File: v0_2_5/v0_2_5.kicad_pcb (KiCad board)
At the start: 2 copper layers, 91.4 x 50.8 mm, 58 parts, among them IC1 RASPBERRY_PI_PICO_W, IC2 BH1750FVI-TR, IC3 AP2138N-3.3TRG1, J1 S2B-PH-SM4-TB_LF__SN_, J2 HYCW110-TF10-180B, J4 SM04B-SRSS-TB, J5 Screw_Terminal_01x03, J6 Conn_01x02_Pin, Q1 DMG2301L-7, Q2 DMG2301L-7, Q3 DMG2301L-7, Q5 DMN3731U-7, U1 AHT20, U2 PCF85063ATL, Y1 Q13FC1350000200

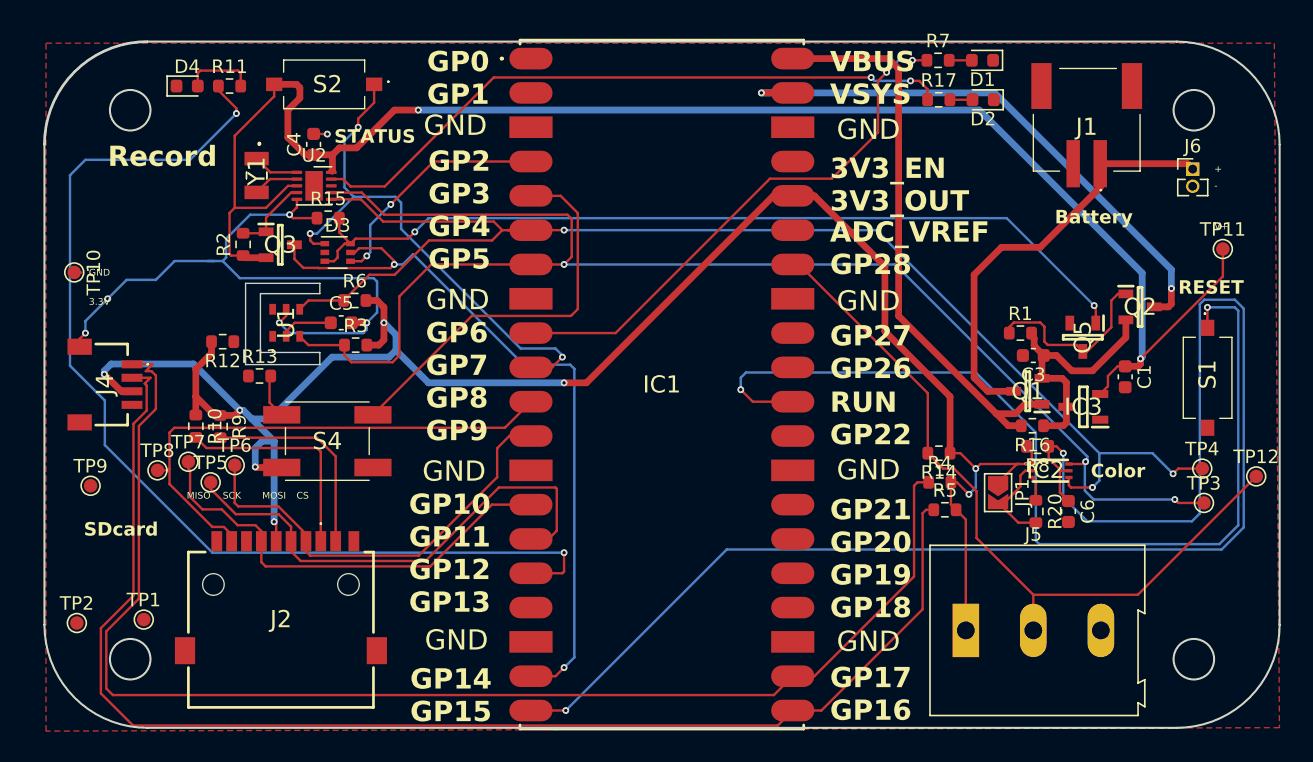
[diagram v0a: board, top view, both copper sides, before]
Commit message: change placement
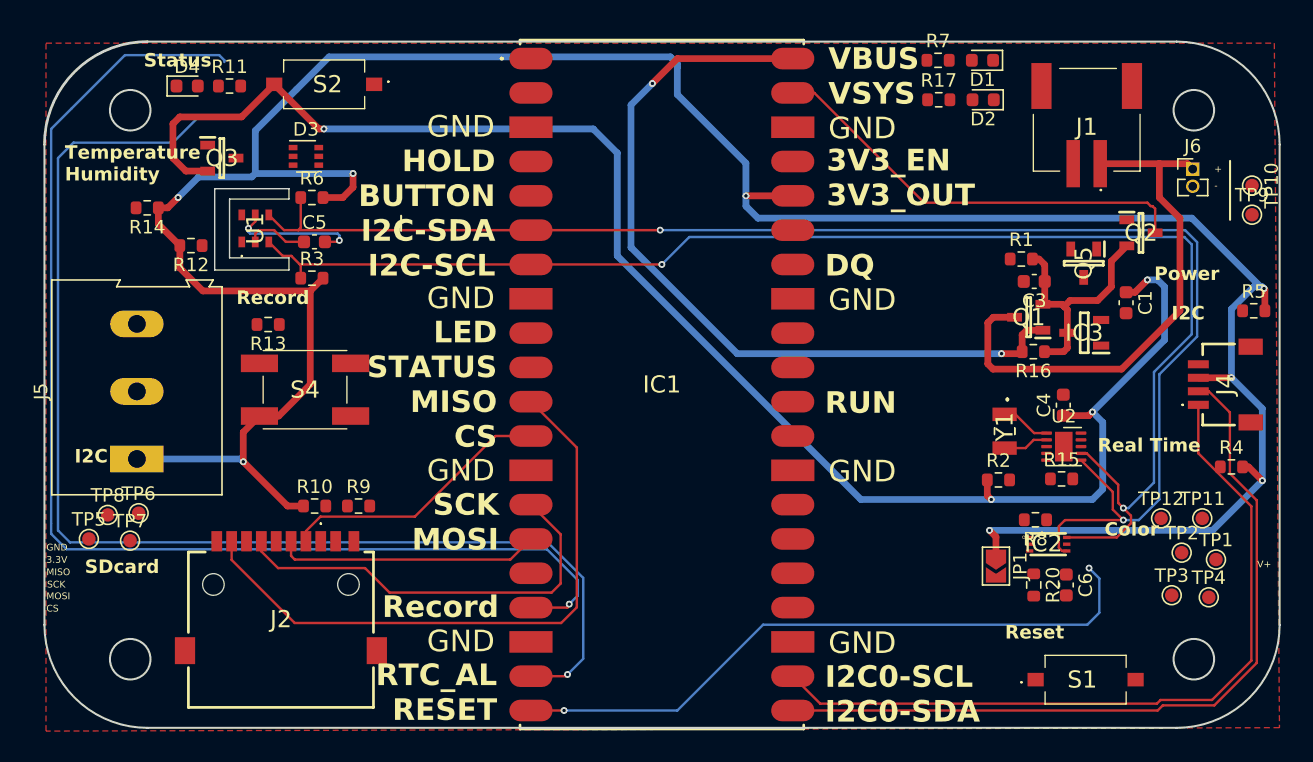
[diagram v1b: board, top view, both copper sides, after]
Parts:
- moved TP9 88.3 mm to (197.0, 15.1)
- moved TP10 87.4 mm to (197.0, 12.9)
- moved J4 83.5 mm to (195.3, 27.6), turned to 90 degrees
- moved TP2 82.0 mm to (191.8, 40.1)
- moved TP1 79.5 mm to (194.4, 40.6)
- moved J5 62.7 mm to (114.5, 33.2), turned to 90 degrees
- moved R14 61.4 mm to (115.2, 14.6)
- moved U2 58.8 mm to (183.1, 32.2)
- moved C4 58.8 mm to (183.0, 29.2)
- moved R2 58.6 mm to (178.2, 34.7), turned to 0 degrees
- moved Y1 58.5 mm to (178.7, 31.1)
- moved R15 57.6 mm to (182.9, 34.6)
- moved R5 27.2 mm to (197.1, 22.2)
- moved S1 24.1 mm to (184.7, 49.5), turned to 0 degrees
- moved R4 21.6 mm to (195.5, 33.7)
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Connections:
- IC1 pad 16: /Record -> unconnected-(IC1-UART0_TX/I2C0_SDA_/SPI1_RX_/GP12-Pad16)
- IC1 pad 17: unconnected-(IC1-UART0_RX/I2C0_SCL_/SPI1_CSN/GP13-Pad17) -> /Record
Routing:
- net /RUN: track 72.4 -> 0.00 mm, vias 2 -> 0
- net /RESET: track 114.7 -> 48.7 mm
- net /VSYS_EN: track 64.8 -> 0.00 mm, vias 2 -> 0
- net +3.3V: track 147.3 -> 205.4 mm
- net /DQ: track 55.3 -> 0.00 mm
- net /ALARM_LED: track 49.0 -> 0.00 mm, vias 2 -> 0
- net GND: track 54.1 -> 9.79 mm, vias 6 -> 2
- net /I2C0_SCL: track 99.4 -> 56.7 mm
- net /I2C0_SDA: track 99.8 -> 58.2 mm
- net /ACT_LED: track 39.9 -> 0.00 mm, vias 2 -> 0
- net /SWITCH_STATUS: track 39.5 -> 0.00 mm, vias 3 -> 0
- net /RTC_ALARM: track 55.5 -> 91.8 mm, vias 2 -> 1
- net /Button: track 29.5 -> 0.00 mm
- net /HOLD_VSYS_EN: track 17.7 -> 0.00 mm, vias 2 -> 0
- net /MOSI: track 37.0 -> 19.6 mm
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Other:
- outline, holes or cut-outs redrawn
- board text added: "DQ"
- board text added: "HOLD BUTTON I2C-SDA I2C-SCL"
- board text added: "I2C"
- board text added: "I2C0-SCL I2C0-SDA"
- board text added: "LED STATUS MISO CS"
- board text added: "Power"
- board text added: "RTC_AL RESET"
- board text added: "Real Time"
- board text added: "Reset"
- board text added: "SCK MOSI"
- board text added: "Status"
- board text added: "Temperature Humidity"
- board text removed: "ADC_VREF"
- board text removed: "Battery"
- board text removed: "GP0 GP1"
- board text removed: "GP10 GP11 GP12 GP13"
- board text removed: "GP14 GP15"
- board text removed: "GP17 GP16"
- board text removed: "GP2 GP3 GP4 GP5"
- board text removed: "GP21 GP20 GP19 GP18"
- board text removed: "GP22"
- board text removed: "GP27 GP26"
- board text removed: "GP28"
- board text removed: "GP6 GP7 GP8 GP9"
- board text removed: "RESET"
- board text removed: "STATUS"
